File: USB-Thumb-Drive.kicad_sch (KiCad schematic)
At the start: 10 parts, among them J101 USB_C_Receptacle_USB2.0_14P, J102 USB_C_Receptacle_USB2.0_14P

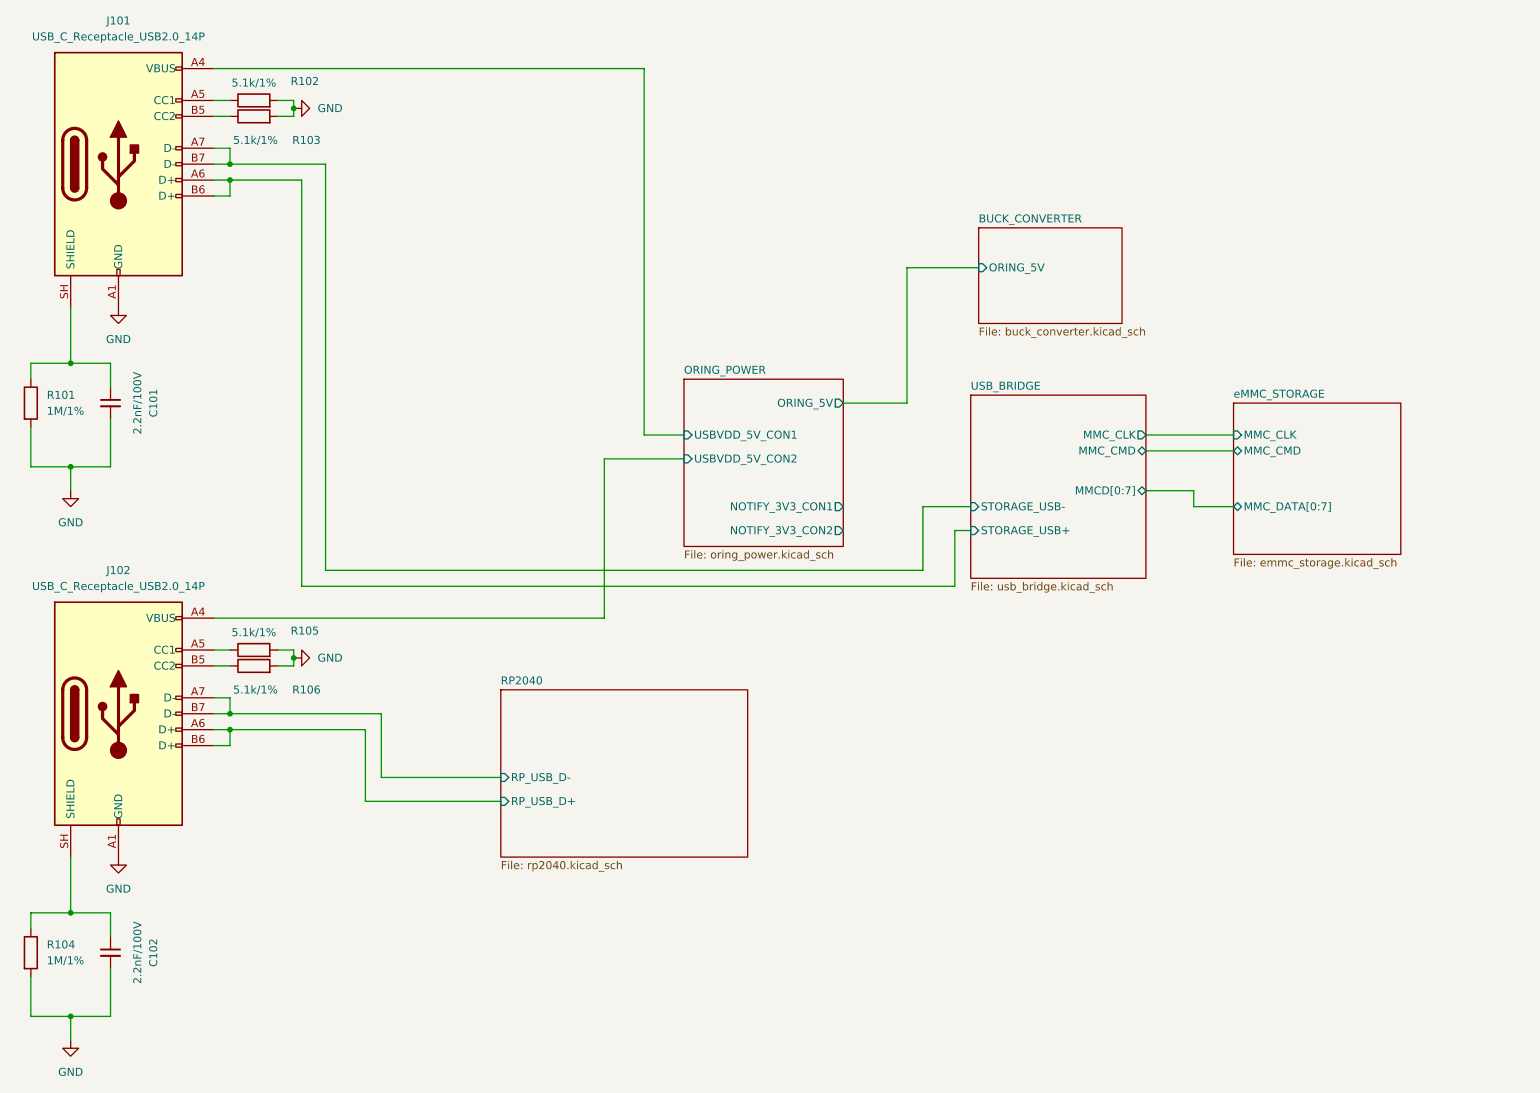
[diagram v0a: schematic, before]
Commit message: avancees majeures sur le schema
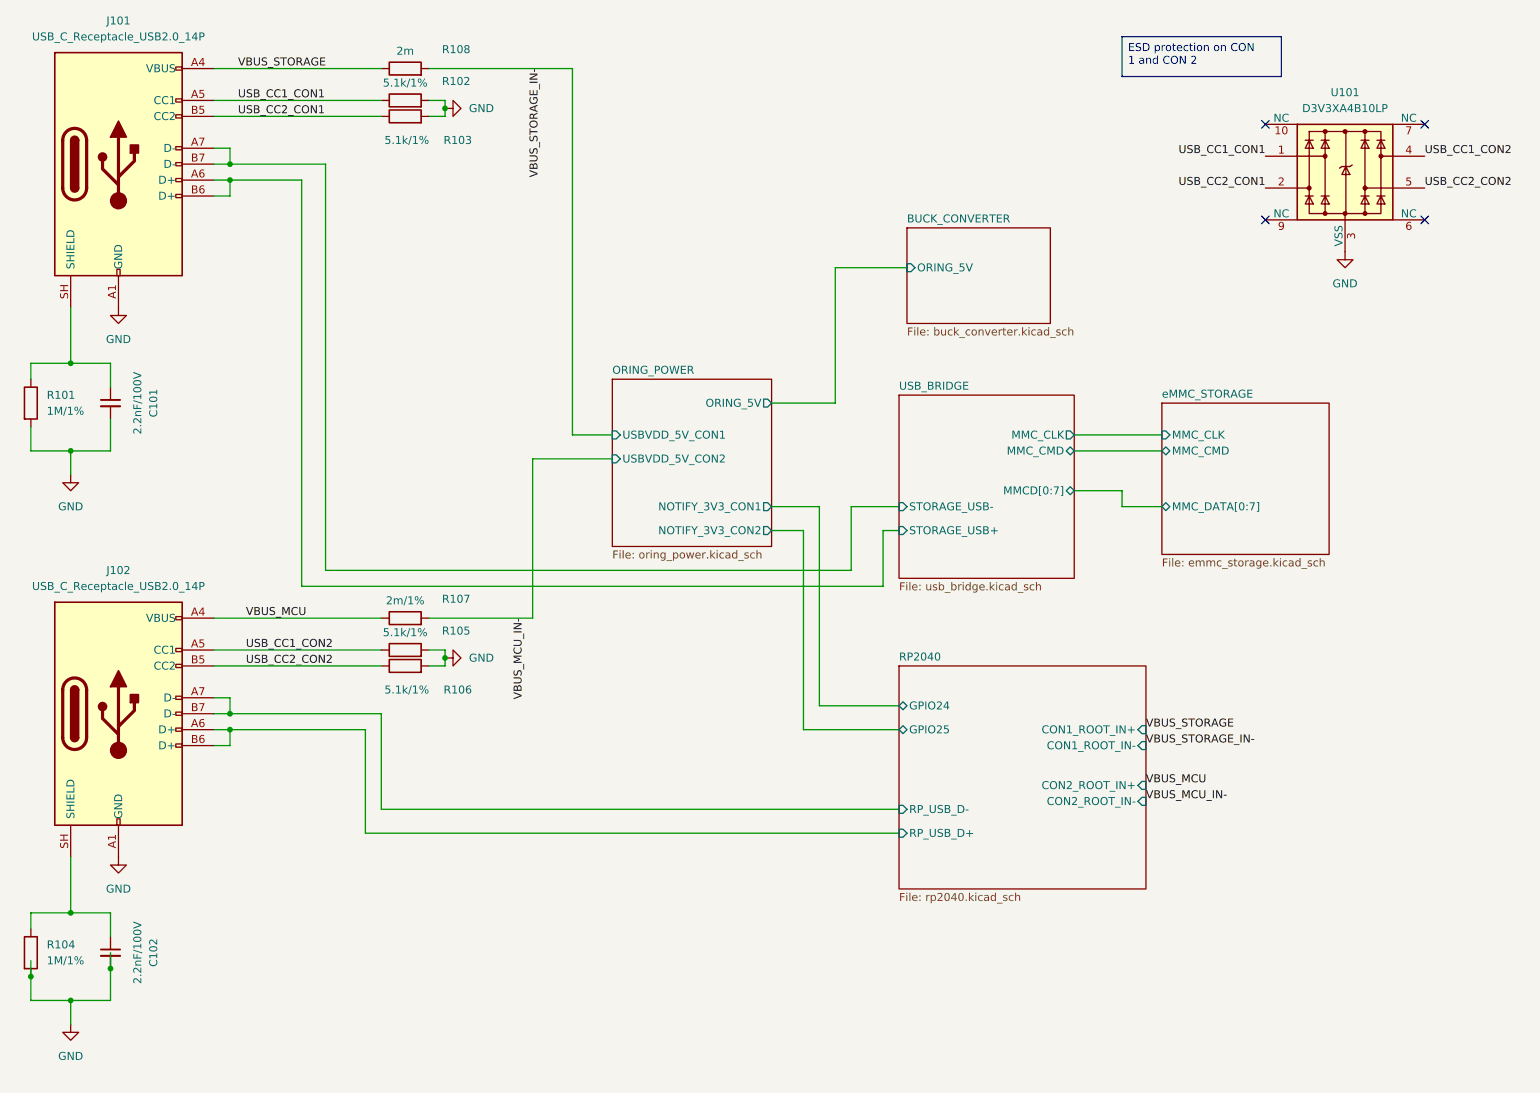
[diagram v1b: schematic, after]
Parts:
- added R107: 2m/1%, Resistor_SMD:R_01005_0402Metric, symbol Device:R
- added R108: 2m, Resistor_SMD:R_01005_0402Metric, symbol Device:R
- added U101: D3V3XA4B10LP, Package_DFN_QFN:Diodes_UDFN-10_1x2.5mm_P0.5mm, symbol Power_Protection:D3V3XA4B10LP
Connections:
- net GND: now also U101.3 (VSS), U101.8 (VSS)
- net USB_CC1_CON1: now reaches J101.A5 (CC1), R102.1
- net USB_CC1_CON1: now also U101.1
- net USB_CC2_CON1: now reaches J101.B5 (CC2), R103.1
- net USB_CC2_CON1: now also U101.2
- net USB_CC1_CON2: now reaches J102.A5 (CC1), R105.1
- net USB_CC1_CON2: now also U101.4
- net USB_CC2_CON2: now reaches J102.B5 (CC2), R106.1
- net USB_CC2_CON2: now also U101.5
- net ORING_POWER/USBVDD_5V_CON1 renamed VBUS_STORAGE
- net VBUS_STORAGE: now also R108.1
- net ORING_POWER/USBVDD_5V_CON2 renamed VBUS_MCU
- net VBUS_MCU: now also R107.1
- new net VBUS_MCU_IN-: R107.2
- new net VBUS_STORAGE_IN-: R108.2
- no-connect marks 0 -> 4
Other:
- sheet RP2040 ports: added CON1_ROOT_IN+, CON1_ROOT_IN-, CON2_ROOT_IN+, CON2_ROOT_IN-, GPIO24, GPIO25; removed none
- moved on the sheet: R102, R103, R105, R106
